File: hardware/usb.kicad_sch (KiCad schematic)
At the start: 5 parts, among them J1 USB_C_Receptacle_USB2.0_16P, U6 TS3USB221

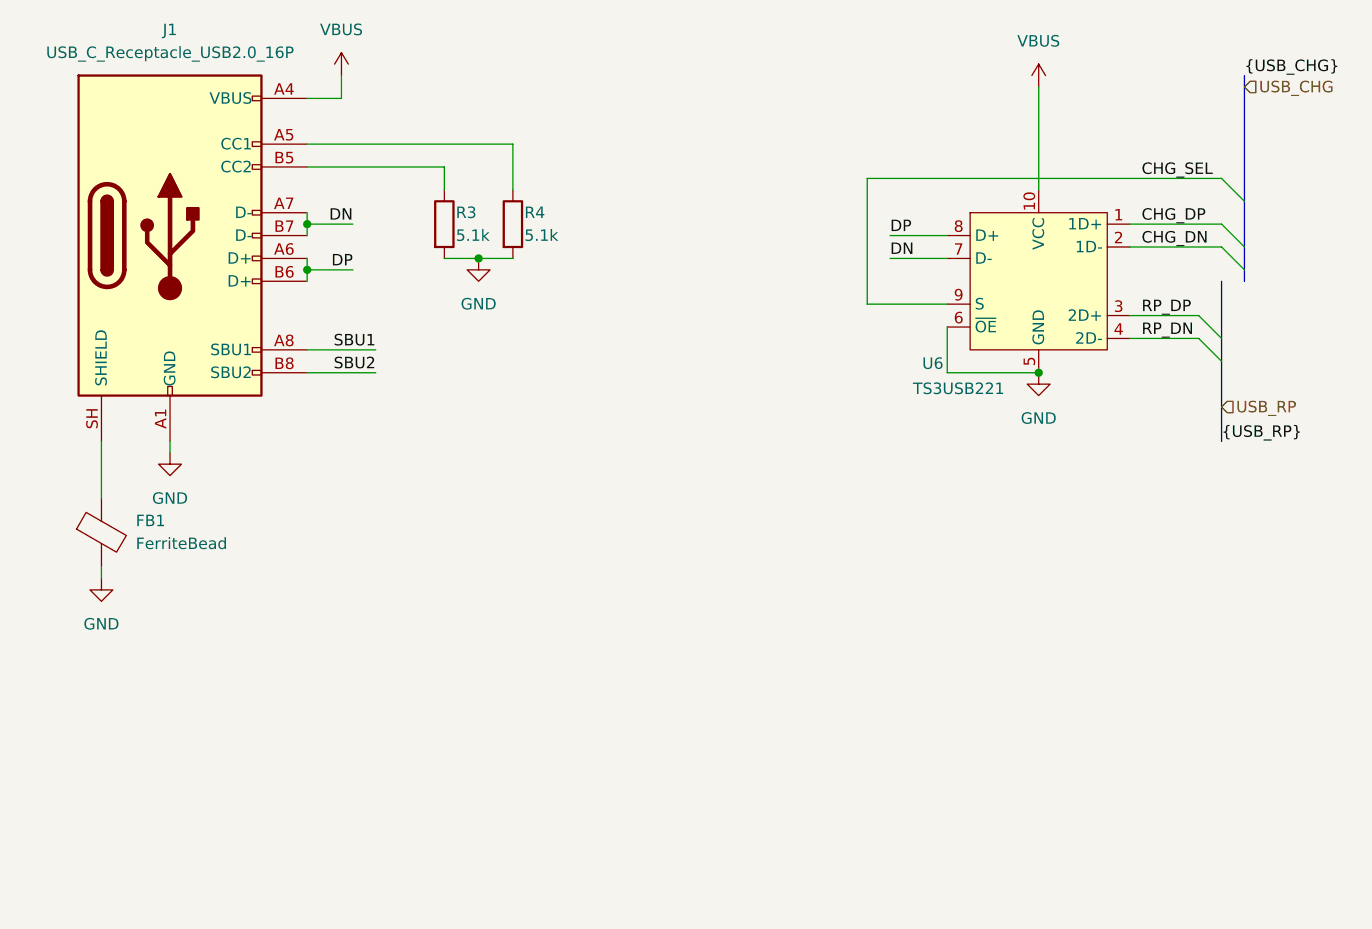
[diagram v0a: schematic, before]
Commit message: charging circuit
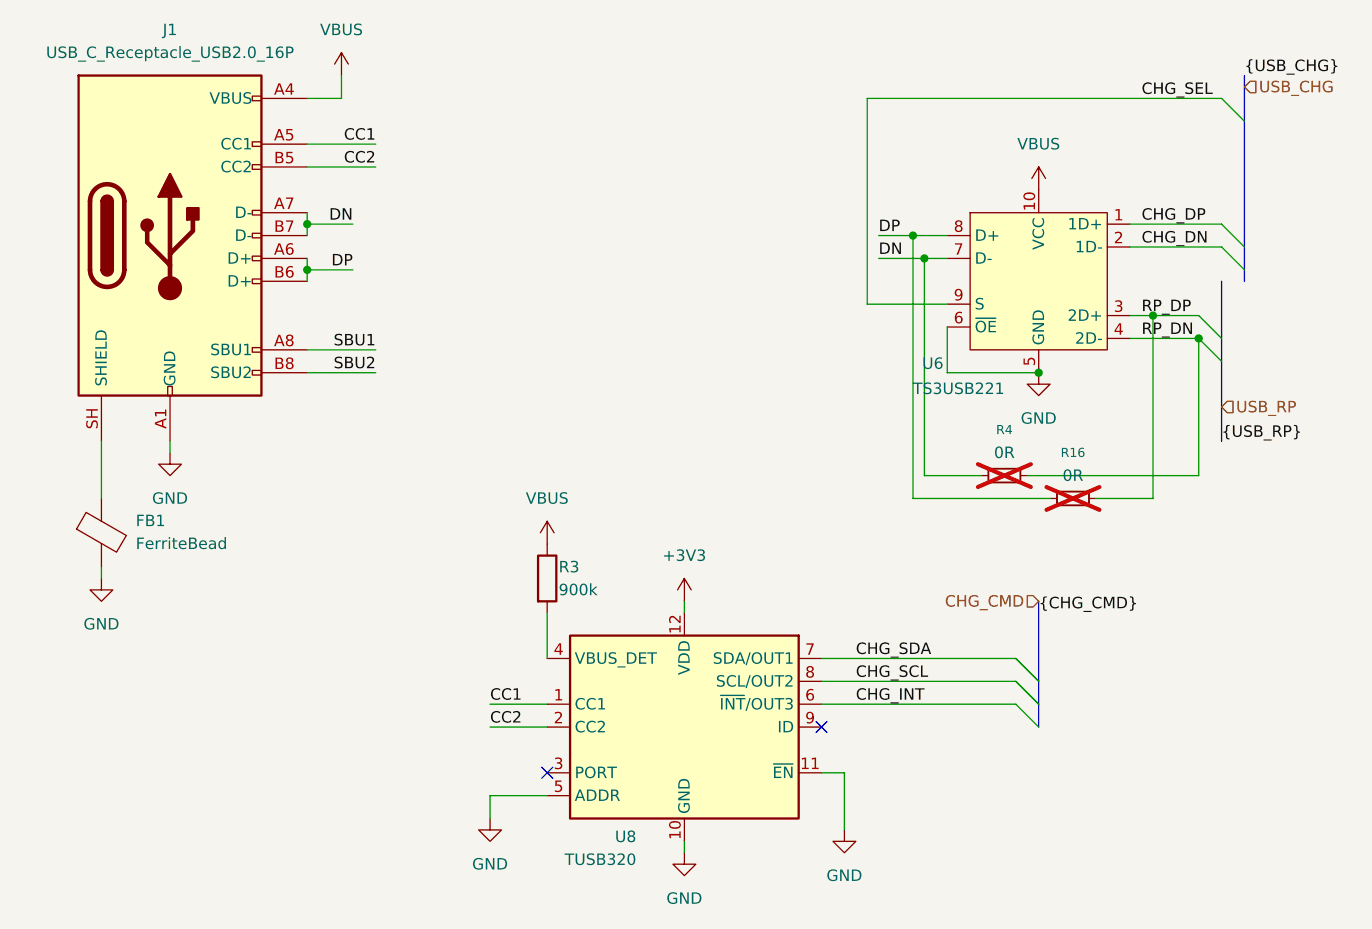
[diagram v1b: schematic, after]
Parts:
- removed R4: 5.1k, symbol Device:R
- added R16, R4: 0R, symbol Device:R_Small
- added U8: TUSB320, Package_DFN_QFN:Texas_X2QFN-12_1.6x1.6mm_P0.4mm, symbol Interface_USB:TUSB320
- R3: value 5.1k -> 900k
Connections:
- net DN: now also R4.1
- net DP: now also R16.1
- net GND: now also U8.10 (GND), U8.11 (~{EN}), U8.5 (ADDR); no longer R3.2
- net RP_DN: now also R4.2
- net RP_DP: now also R16.2
- net VBUS: now also R3.1
- net CC2: now reaches J1.B5 (CC2)
- net CC2: now also U8.2 (CC2); no longer R3.1
- net CC1: now reaches J1.A5 (CC1)
- net CC1: now also U8.1 (CC1)
- new net: R3.2, U8.4 (VBUS_DET)
- new net +3V3: U8.12 (VDD)
- new net CHG_INT: U8.6 (~{INT}/OUT3)
- new net CHG_SCL: U8.8 (SCL/OUT2)
- new net CHG_SDA: U8.7 (SDA/OUT1)
- no-connect marks 0 -> 2
